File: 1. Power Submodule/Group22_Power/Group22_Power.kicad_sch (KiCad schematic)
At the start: 9 parts

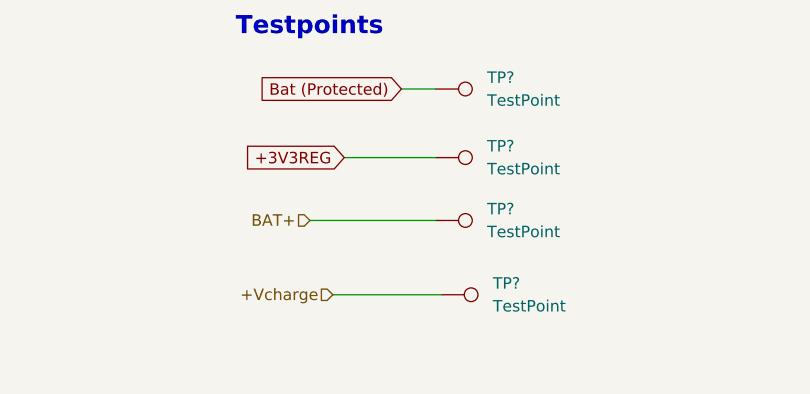
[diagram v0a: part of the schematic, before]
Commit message: $1
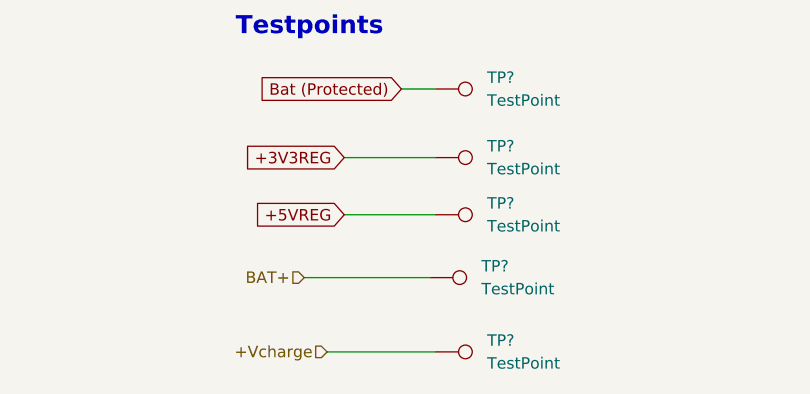
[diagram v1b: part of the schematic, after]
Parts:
- added TP?: TestPoint, TestPoint:TestPoint_Pad_D2.0mm, symbol Connector:TestPoint
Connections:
- new net +5VREG: TP?.1
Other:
- moved on the sheet: TP?
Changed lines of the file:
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@@
     (stroke (width 0) (type default) (color 0 0 0 0))
   )
-  (wire (pts (xy 69.85 160.02) (xy 81.915 160.02))
+  (wire (pts (xy 69.215 166.37) (xy 81.28 166.37))
     (stroke (width 0) (type default) (color 0 0 0 0))
   )
@@
     (stroke (width 0) (type default) (color 0 0 0 0))
   )
-  (wire (pts (xy 67.31 151.765) (xy 81.28 151.765))
+  (wire (pts (xy 66.675 158.115) (xy 80.645 158.115))
     (stroke (width 0) (type default) (color 0 0 0 0))
   )
@@
   )
   (wire (pts (xy 77.47 137.16) (xy 81.28 137.16))
+    (stroke (width 0) (type default) (color 0 0 0 0))
+  )
+  (wire (pts (xy 71.12 151.13) (xy 81.28 151.13))
     (stroke (width 0) (type default) (color 0 0 0 0))
   )
@@
     (effects (font (size 2.0066 2.0066) (thickness 0.4013) bold) (justify left bottom))
   )
+  (global_label "+5VREG" (shape input) (at 71.12 151.13 180) (fields_autoplaced)
+    (effects (font (size 1.27 1.27)) (justify right))
+    (property "Intersheet References" "${INTERSHEET_REFS}" (id 0) (at 61.1474 151.0506 0)
+      (effects (font (size 1.27 1.27)) (justify right) hide)
+    )
+  )
   (global_label "+3V3REG" (shape input) (at 71.12 144.78 180) (fields_autoplaced)
     (effects (font (size 1.27 1.27)) (justify right))
@@
     (effects (font (size 1.27 1.27)) (justify left))
   )
-  (hierarchical_label "BAT+" (shape input) (at 67.31 151.765 180)
-    (effects (font (size 1.27 1.27)) (justify right))
-  )
-  (hierarchical_label "+Vcharge" (shape input) (at 69.85 160.02 180)
+  (hierarchical_label "BAT+" (shape input) (at 66.675 158.115 180)
+    (effects (font (size 1.27 1.27)) (justify right))
+  )
+  (hierarchical_label "+Vcharge" (shape input) (at 69.215 166.37 180)
     (effects (font (size 1.27 1.27)) (justify right))
   )
@@
     (pin "2")
   )
-  (symbol (lib_id "Connector:TestPoint") (at 81.915 160.02 270) (unit 1)
-    (in_bom yes) (on_board yes) (fields_autoplaced)
-    (property "Reference" "TP?" (id 0) (at 87.63 158.7499 90)
-      (effects (font (size 1.27 1.27)) (justify left))
-    )
-    (property "Value" "TestPoint" (id 1) (at 87.63 161.2899 90)
-      (effects (font (size 1.27 1.27)) (justify left))
-    )
-    (property "Footprint" "TestPoint:TestPoint_Pad_D2.0mm" (id 2) (at 81.915 165.1 0)
-      (effects (font (size 1.27 1.27)) hide)
-    )
-    (property "Datasheet" "~" (id 3) (at 81.915 165.1 0)
-      (effects (font (size 1.27 1.27)) hide)
-    )
-    (pin "1")
-  )
-  (symbol (lib_id "Connector:TestPoint") (at 81.28 151.765 270) (unit 1)
-    (in_bom yes) (on_board yes) (fields_autoplaced)
-    (property "Reference" "TP?" (id 0) (at 86.995 150.4949 90)
-      (effects (font (size 1.27 1.27)) (justify left))
-    )
-    (property "Value" "TestPoint" (id 1) (at 86.995 153.0349 90)
-      (effects (font (size 1.27 1.27)) (justify left))
-    )
-    (property "Footprint" "TestPoint:TestPoint_Pad_D2.0mm" (id 2) (at 81.28 156.845 0)
-      (effects (font (size 1.27 1.27)) hide)
-    )
-    (property "Datasheet" "~" (id 3) (at 81.28 156.845 0)
+  (symbol (lib_id "Connector:TestPoint") (at 81.28 166.37 270) (unit 1)
+    (in_bom yes) (on_board yes) (fields_autoplaced)
+    (property "Reference" "TP?" (id 0) (at 86.995 165.0999 90)
+      (effects (font (size 1.27 1.27)) (justify left))
+    )
+    (property "Value" "TestPoint" (id 1) (at 86.995 167.6399 90)
+      (effects (font (size 1.27 1.27)) (justify left))
+    )
+    (property "Footprint" "TestPoint:TestPoint_Pad_D2.0mm" (id 2) (at 81.28 171.45 0)
+      (effects (font (size 1.27 1.27)) hide)
+    )
+    (property "Datasheet" "~" (id 3) (at 81.28 171.45 0)
+      (effects (font (size 1.27 1.27)) hide)
+    )
+    (pin "1")
+  )
+  (symbol (lib_id "Connector:TestPoint") (at 80.645 158.115 270) (unit 1)
+    (in_bom yes) (on_board yes) (fields_autoplaced)
+    (property "Reference" "TP?" (id 0) (at 86.36 156.8449 90)
+      (effects (font (size 1.27 1.27)) (justify left))
+    )
+    (property "Value" "TestPoint" (id 1) (at 86.36 159.3849 90)
+      (effects (font (size 1.27 1.27)) (justify left))
+    )
+    (property "Footprint" "TestPoint:TestPoint_Pad_D2.0mm" (id 2) (at 80.645 163.195 0)
+      (effects (font (size 1.27 1.27)) hide)
+    )
+    (property "Datasheet" "~" (id 3) (at 80.645 163.195 0)
+      (effects (font (size 1.27 1.27)) hide)
+    )
+    (pin "1")
+  )
+  (symbol (lib_id "Connector:TestPoint") (at 81.28 151.13 270) (unit 1)
+    (in_bom yes) (on_board yes) (fields_autoplaced)
+    (property "Reference" "TP?" (id 0) (at 86.995 149.8599 90)
+      (effects (font (size 1.27 1.27)) (justify left))
+    )
+    (property "Value" "TestPoint" (id 1) (at 86.995 152.3999 90)
+      (effects (font (size 1.27 1.27)) (justify left))
+    )
+    (property "Footprint" "TestPoint:TestPoint_Pad_D2.0mm" (id 2) (at 81.28 156.21 0)
+      (effects (font (size 1.27 1.27)) hide)
+    )
+    (property "Datasheet" "~" (id 3) (at 81.28 156.21 0)
       (effects (font (size 1.27 1.27)) hide)
     )
@@
       (reference "#PWR?") (unit 1) (value "GND") (footprint "")
     )
+    (path "/ba90ddbb-a325-41f6-b0d8-c98df51ea380/8d6d3835-c3f2-49ba-8734-2d047f1828fb"
+      (reference "#PWR?") (unit 1) (value "GND") (footprint "")
+    )
+    (path "/ba90ddbb-a325-41f6-b0d8-c98df51ea380/982f84ae-47e5-4fd9-a9be-14d67166ac27"
+      (reference "#PWR?") (unit 1) (value "GND") (footprint "")
+    )
     (path "/ba90ddbb-a325-41f6-b0d8-c98df51ea380/9ce7d0da-35e3-40ba-b4d8-e3757a9f675d"
       (reference "#PWR?") (unit 1) (value "GND") (footprint "")
     )
+    (path "/ba90ddbb-a325-41f6-b0d8-c98df51ea380/c341da05-6a33-4f59-a518-6c3562d778f2"
+      (reference "#PWR?") (unit 1) (value "GND") (footprint "")
+    )
     (path "/c56c35c5-fd2c-4ef4-a40c-984e0dbbe493"
       (reference "#PWR?") (unit 1) (value "GND") (footprint "")
     )
     (path "/ba90ddbb-a325-41f6-b0d8-c98df51ea380/ce39ddfd-7976-4151-87a8-8cb3460c8c08"
+      (reference "#PWR?") (unit 1) (value "GND") (footprint "")
+    )
+    (path "/ba90ddbb-a325-41f6-b0d8-c98df51ea380/ff18062c-e585-484f-89dc-9ab747ac9cf8"
       (reference "#PWR?") (unit 1) (value "GND") (footprint "")
     )
@@
       (reference "C?") (unit 1) (value "10u") (footprint "Project_Library:10uF Cap")
     )
+    (path "/ba90ddbb-a325-41f6-b0d8-c98df51ea380/37ad02bc-6583-40d7-bfd4-0fccea7b6dd7"
+      (reference "C?") (unit 1) (value "100n") (footprint "Capacitor_SMD:C_0603_1608Metric")
+    )
+    (path "/ba90ddbb-a325-41f6-b0d8-c98df51ea380/523c304d-a582-4843-bb4a-26405d544ebb"
+      (reference "C?") (unit 1) (value "100n") (footprint "Capacitor_SMD:C_0603_1608Metric")
+    )
+    (path "/ba90ddbb-a325-41f6-b0d8-c98df51ea380/aa315501-8985-4f50-993e-d2a92acb69d5"
+      (reference "C?") (unit 1) (value "100n") (footprint "Capacitor_SMD:C_0603_1608Metric")
+    )
     (path "/c7b32c44-c58e-418a-929d-90ece0ff7a01"
       (reference "C?") (unit 1) (value "1u") (footprint "Project_Library:1uF Cap")
@@
       (reference "D?") (unit 1) (value "Diode") (footprint "Project_Library:Schottky Diode")
     )
+    (path "/ba90ddbb-a325-41f6-b0d8-c98df51ea380/9b4abebb-cd1f-468c-ae5e-004b19b4ac21"
+      (reference "J?") (unit 1) (value "Conn_01x02_Male") (footprint "")
+    )
     (path "/ba90ddbb-a325-41f6-b0d8-c98df51ea380/c6ac832d-338e-49e9-a749-70fe953af321"
       (reference "J?") (unit 1) (value "Conn_01x02_Male") (footprint "Connector_PinHeader_2.54mm:PinHeader_1x02_P2.54mm_Vertical")
@@
       (reference "TP?") (unit 1) (value "TestPoint") (footprint "TestPoint:TestPoint_Pad_D2.0mm")
     )
+    (path "/bed859c1-79d1-431d-8430-6c1171048f0f"
+      (reference "TP?") (unit 1) (value "TestPoint") (footprint "TestPoint:TestPoint_Pad_D2.0mm")
+    )
     (path "/faf22fdc-9e02-4ec2-89cb-298aa5fdd5f3"
       (reference "TP?") (unit 1) (value "TestPoint") (footprint "TestPoint:TestPoint_Pad_D2.0mm")
@@
     )
     (path "/ba90ddbb-a325-41f6-b0d8-c98df51ea380/4a12ae86-257a-4133-974c-c8c55838862f"
-      (reference "U?") (unit 1) (value "HT75") (footprint "Project_Library:HT75")
-    )
-  )
+      (reference "U?") (unit 1) (value "XC6206") (footprint "Package_TO_SOT_SMD:SOT-23")
+    )
+    (path "/ba90ddbb-a325-41f6-b0d8-c98df51ea380/81efe728-ae5e-45ab-88e5-6b9aa2c0510b"
+      (reference "U?") (unit 1) (value "L78M") (footprint "Package_TO_SOT_SMD:TO-252-2")
+    )
+  )
